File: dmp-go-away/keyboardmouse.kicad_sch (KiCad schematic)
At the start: 7 parts, among them J3 Keyboard, J4 Mouse, U1 M6117C

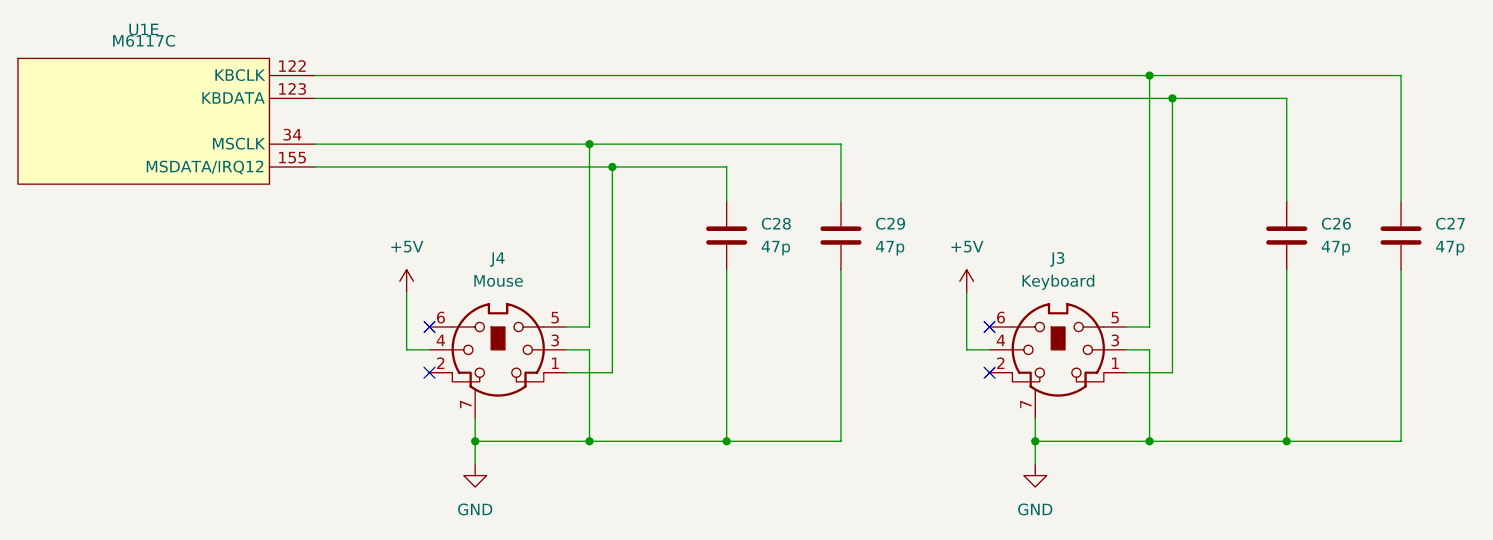
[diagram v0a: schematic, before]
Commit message: Adding layout of dmp-go-away in progress
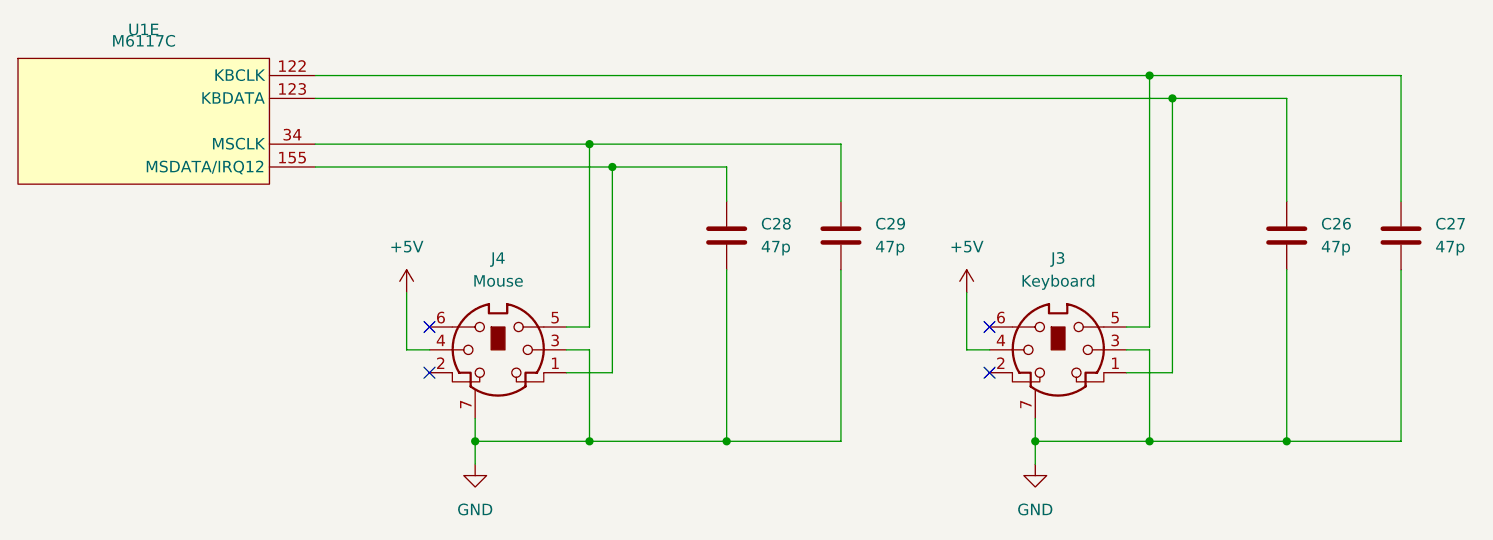
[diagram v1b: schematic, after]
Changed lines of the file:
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@@
 (kicad_sch
-	(version 20231120)
+	(version 20250114)
 	(generator "eeschema")
-	(generator_version "8.0")
+	(generator_version "9.0")
 	(paper "USLetter")
 	(junction
